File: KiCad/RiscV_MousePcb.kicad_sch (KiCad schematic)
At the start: 46 parts, among them J1 Conn_01x04_Pin, U1 TLV70019_SOT23-5, U2 MIC5219-3.3YM5, U3 CH32V30xRxTx, U4 TPD2EUSB30, U5 TPD2EUSB30, U6 TPD2EUSB30, Y1 8MHZ_CMOS

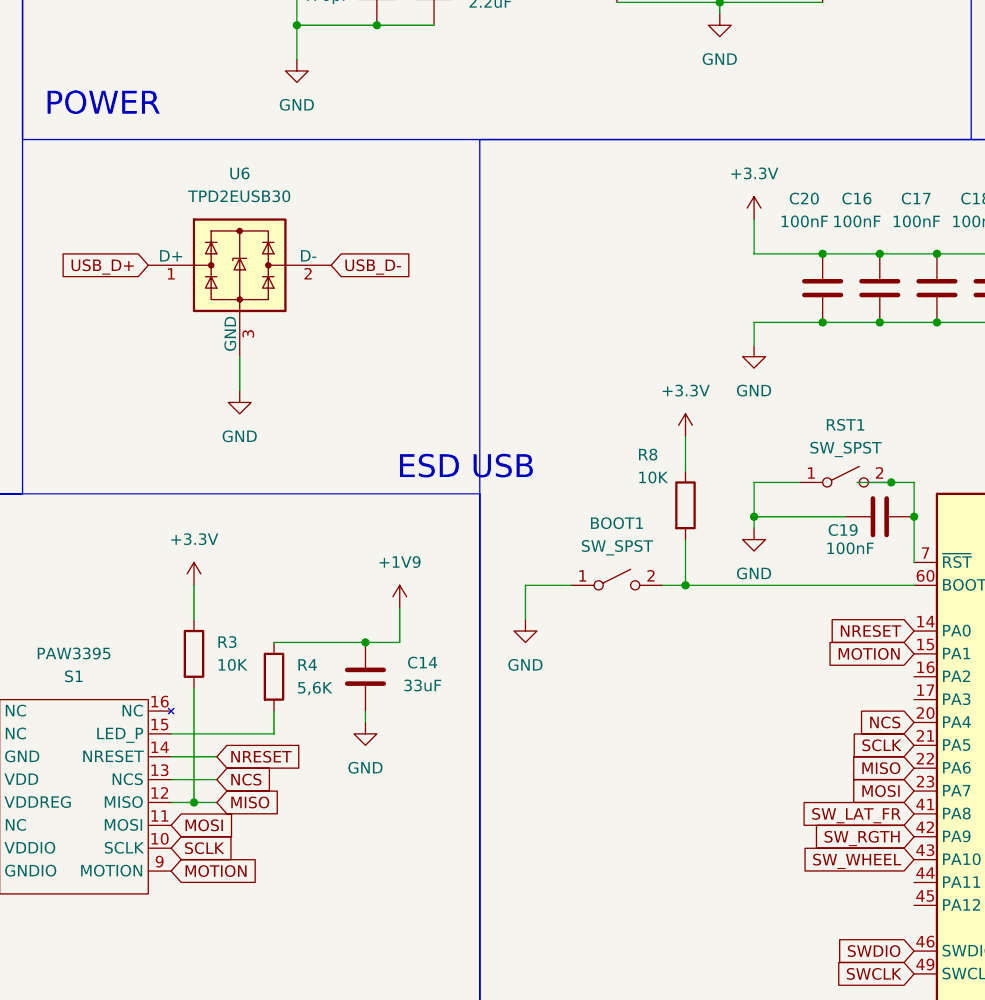
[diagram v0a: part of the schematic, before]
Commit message: Add files via upload
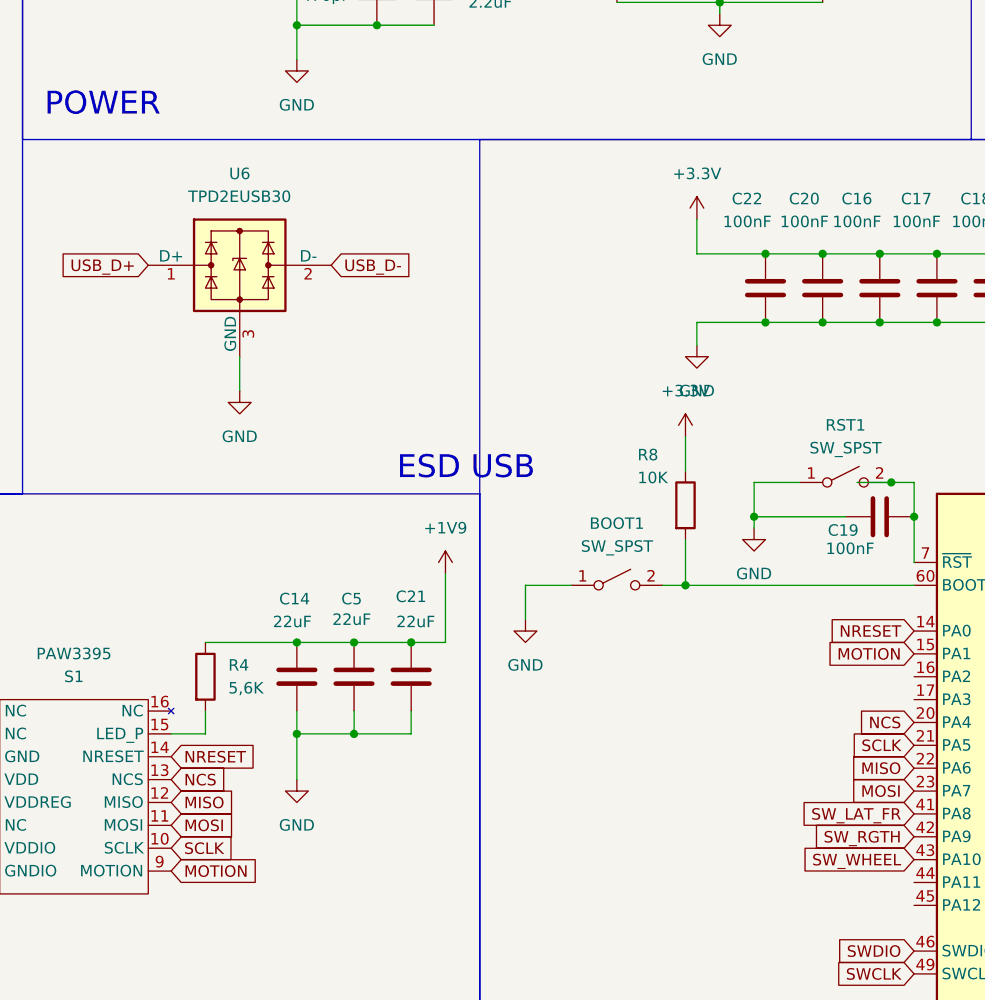
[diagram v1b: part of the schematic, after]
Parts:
- removed R3: 10K, Capacitor_SMD:C_0603_1608Metric, symbol Device:R
- added C21, C5: 22uF, Capacitor_SMD:C_0805_2012Metric_Pad1.18x1.45mm_HandSolder, symbol Device:C
- added C22: 100nF, Capacitor_SMD:C_0805_2012Metric_Pad1.18x1.45mm_HandSolder, symbol Device:C
- C1: footprint Capacitor_SMD:C_0603_1608Metric -> Capacitor_SMD:C_0805_2012Metric_Pad1.18x1.45mm_HandSolder
- C10, C11, C12, C13, C15, C16, C17, C18, C19, C2, C20, C3, C4, C6, C7, C8, C9: footprint Capacitor_SMD:C_0402_1005Metric -> Capacitor_SMD:C_0805_2012Metric_Pad1.18x1.45mm_HandSolder
- C14: value 33uF -> 22uF; footprint Capacitor_SMD:C_0402_1005Metric -> Capacitor_SMD:C_0805_2012Metric_Pad1.18x1.45mm_HandSolder
- R4, R5, R6, R7, R8, R9: footprint Capacitor_SMD:C_0603_1608Metric -> Resistor_SMD:R_0805_2012Metric_Pad1.20x1.40mm_HandSolder
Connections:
- net +1V9: now also C21.2, C5.2
- net +3.3V: now also C22.1
- net GND: now also C21.1, C22.2, C5.1
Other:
- moved on the sheet: C14, R4
